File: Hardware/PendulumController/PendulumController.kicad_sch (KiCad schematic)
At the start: 24 parts, among them J101 MOTOR, J102 ENCODER, Q101 MMBT3904, Q102 MMBT3906

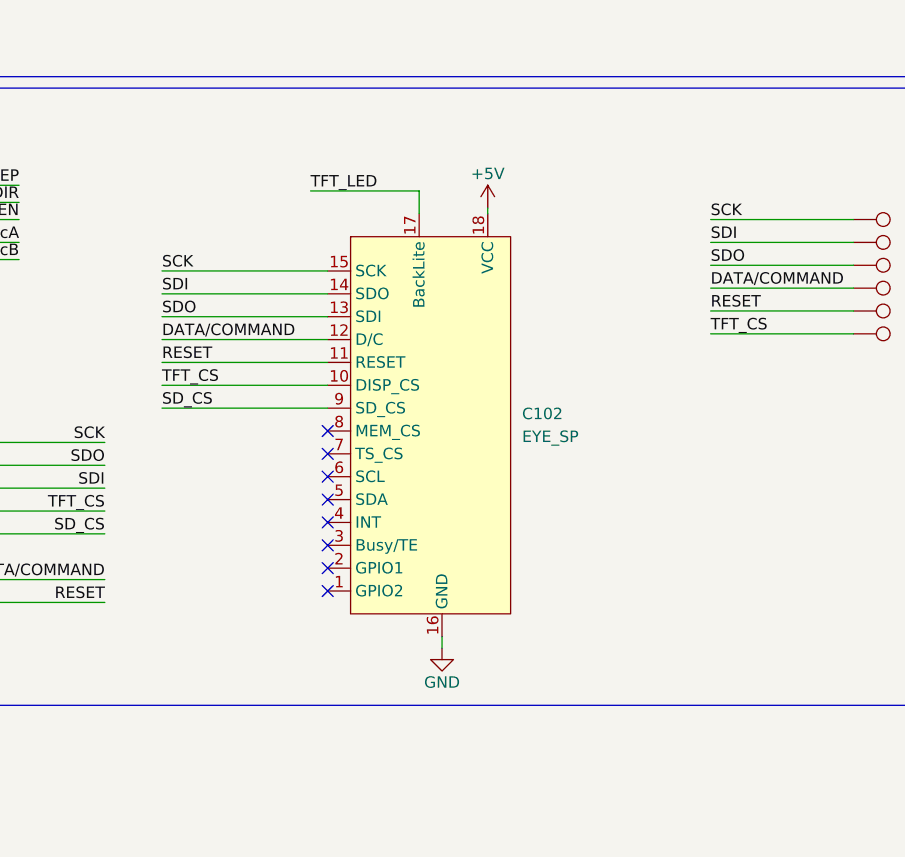
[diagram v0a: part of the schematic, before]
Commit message: Firmware (#15)
Merged for PRR
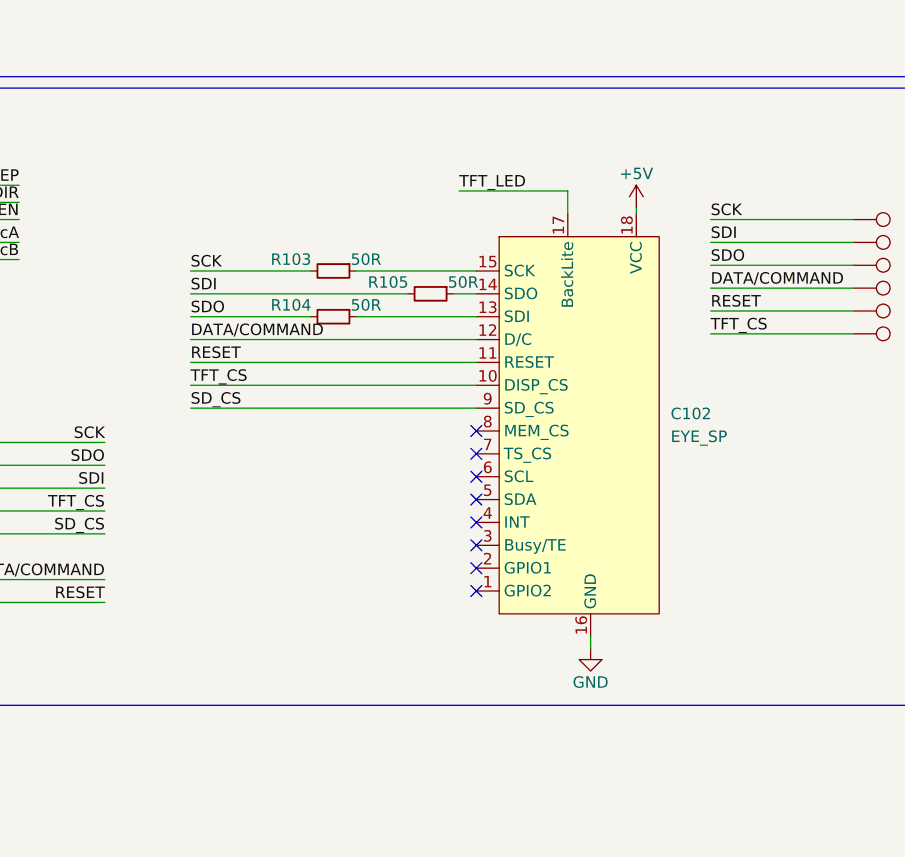
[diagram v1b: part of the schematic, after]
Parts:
- added R103, R104, R105: 50R, Resistor_SMD:R_0805_2012Metric, symbol Device:R_Small
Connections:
- net SCK: now also R103.2; no longer C102.15 (SCK)
- net SDI: now also R105.2; no longer C102.14 (SDO)
- net SDO: now also R104.2; no longer C102.13 (SDI)
- new net: C102.15 (SCK), R103.1
- new net: C102.13 (SDI), R104.1
- new net: C102.14 (SDO), R105.1
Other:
- moved on the sheet: C102
